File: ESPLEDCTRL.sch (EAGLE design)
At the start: 5 parts, among them J1 22-27-2031-03, X3 ZX62D-B-5PA8

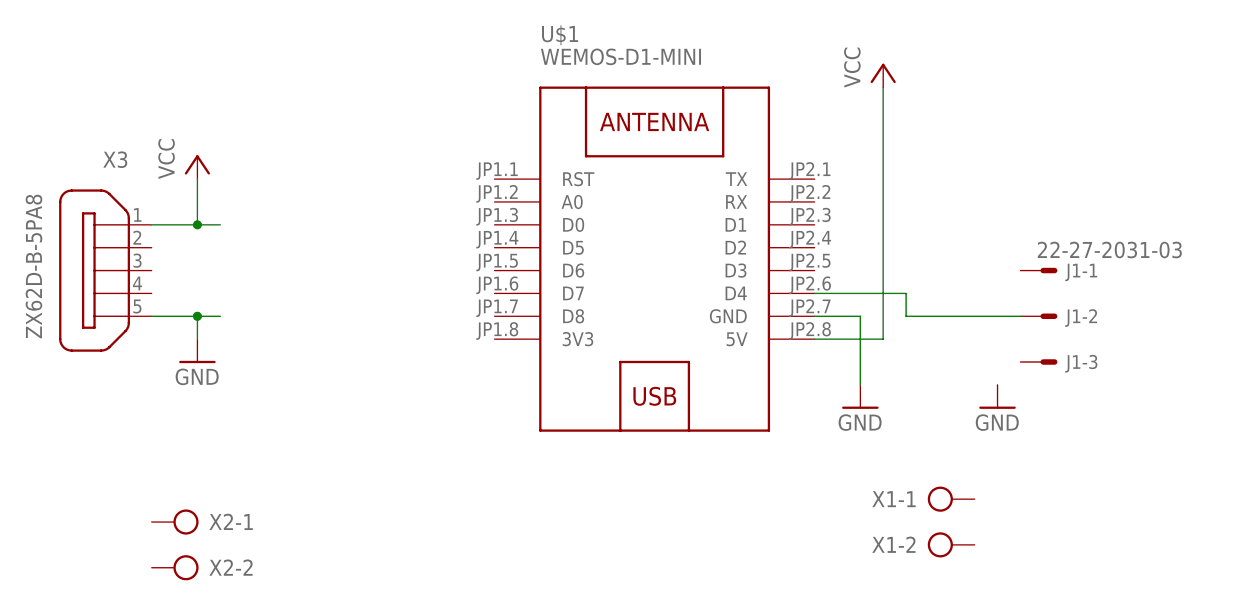
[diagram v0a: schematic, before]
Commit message: bla
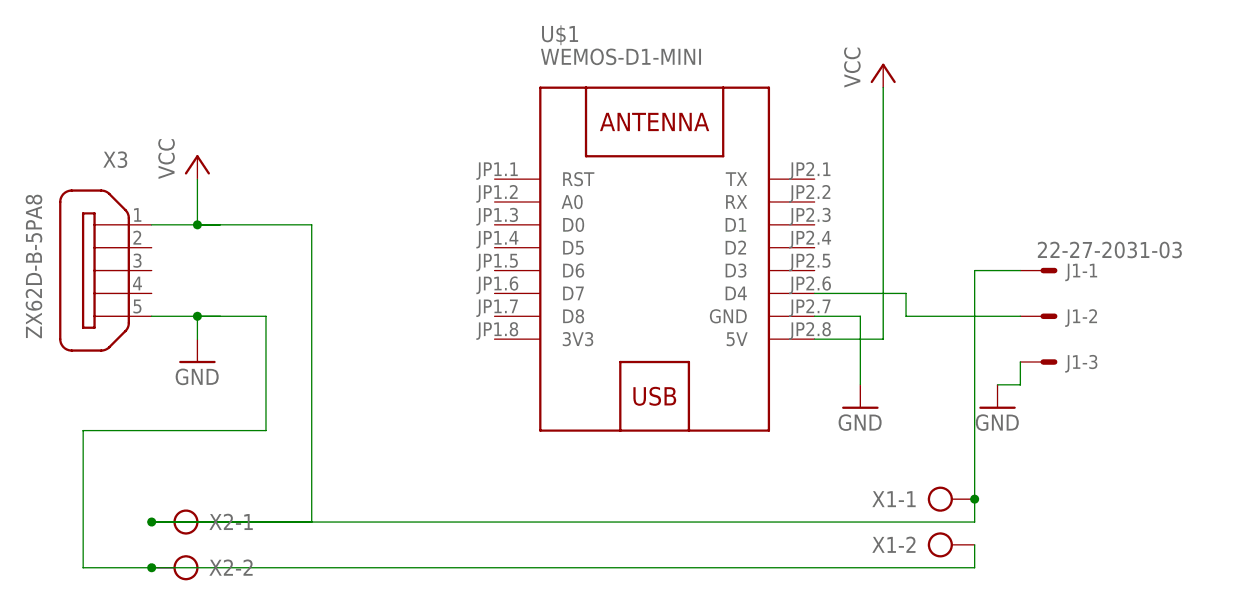
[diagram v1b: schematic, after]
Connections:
- net GND: now also J1-3.S, X1-2.KL, X2-2.KL
- net VCC: now also J1-1.S, X1-1.KL, X2-1.KL
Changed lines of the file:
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@@
 <?xml version="1.0" encoding="utf-8"?>
 <!DOCTYPE eagle SYSTEM "eagle.dtd">
-<eagle version="8.7.1">
+<eagle version="9.5.1">
 <drawing>
 <settings>
@@
 </plain>
 <instances>
-<instance part="X3" gate="G$1" x="27.94" y="58.42" rot="MR0"/>
-<instance part="P+1" gate="VCC" x="38.1" y="71.12"/>
-<instance part="GND1" gate="1" x="38.1" y="48.26"/>
-<instance part="U$1" gate="G$1" x="88.9" y="58.42"/>
-<instance part="X1" gate="-1" x="119.38" y="33.02"/>
-<instance part="X1" gate="-2" x="119.38" y="27.94"/>
-<instance part="X2" gate="-1" x="38.1" y="30.48" rot="MR0"/>
-<instance part="X2" gate="-2" x="38.1" y="25.4" rot="MR0"/>
-<instance part="J1" gate="-1" x="132.08" y="58.42"/>
-<instance part="J1" gate="-2" x="132.08" y="53.34"/>
-<instance part="J1" gate="-3" x="132.08" y="48.26"/>
-<instance part="GND2" gate="1" x="127" y="43.18"/>
-<instance part="P+2" gate="VCC" x="114.3" y="81.28"/>
-<instance part="GND3" gate="1" x="111.76" y="43.18"/>
+<instance part="X3" gate="G$1" x="27.94" y="58.42" smashed="yes" rot="MR0">
+<attribute name="NAME" x="30.48" y="69.85" size="1.778" layer="95" font="vector" rot="MR0"/>
+<attribute name="VALUE" x="19.05" y="50.8" size="1.778" layer="96" font="vector" rot="MR90"/>
+</instance>
+<instance part="P+1" gate="VCC" x="38.1" y="71.12" smashed="yes">
+<attribute name="VALUE" x="35.56" y="68.58" size="1.778" layer="96" rot="R90"/>
+</instance>
+<instance part="GND1" gate="1" x="38.1" y="48.26" smashed="yes">
+<attribute name="VALUE" x="35.56" y="45.72" size="1.778" layer="96"/>
+</instance>
+<instance part="U$1" gate="G$1" x="88.9" y="58.42" smashed="yes">
+<attribute name="NAME" x="76.2" y="83.82" size="1.778" layer="95"/>
+<attribute name="VALUE" x="76.2" y="81.28" size="1.778" layer="96"/>
+</instance>
+<instance part="X1" gate="-1" x="119.38" y="33.02" smashed="yes">
+<attribute name="NAME" x="118.11" y="33.909" size="1.778" layer="95" rot="R180"/>
+</instance>
+<instance part="X1" gate="-2" x="119.38" y="27.94" smashed="yes">
+<attribute name="NAME" x="118.11" y="28.829" size="1.778" layer="95" rot="R180"/>
+<attribute name="VALUE" x="115.57" y="24.257" size="1.778" layer="96"/>
+</instance>
+<instance part="X2" gate="-1" x="38.1" y="30.48" smashed="yes" rot="MR0">
+<attribute name="NAME" x="39.37" y="31.369" size="1.778" layer="95" rot="MR180"/>
+</instance>
+<instance part="X2" gate="-2" x="38.1" y="25.4" smashed="yes" rot="MR0">
+<attribute name="NAME" x="39.37" y="26.289" size="1.778" layer="95" rot="MR180"/>
+<attribute name="VALUE" x="41.91" y="21.717" size="1.778" layer="96" rot="MR0"/>
+</instance>
+<instance part="J1" gate="-1" x="132.08" y="58.42" smashed="yes">
+<attribute name="NAME" x="134.62" y="57.658" size="1.524" layer="95"/>
+<attribute name="VALUE" x="131.318" y="59.817" size="1.778" layer="96"/>
+</instance>
+<instance part="J1" gate="-2" x="132.08" y="53.34" smashed="yes">
+<attribute name="NAME" x="134.62" y="52.578" size="1.524" layer="95"/>
+</instance>
+<instance part="J1" gate="-3" x="132.08" y="48.26" smashed="yes">
+<attribute name="NAME" x="134.62" y="47.498" size="1.524" layer="95"/>
+</instance>
+<instance part="GND2" gate="1" x="127" y="43.18" smashed="yes">
+<attribute name="VALUE" x="124.46" y="40.64" size="1.778" layer="96"/>
+</instance>
+<instance part="P+2" gate="VCC" x="114.3" y="81.28" smashed="yes">
+<attribute name="VALUE" x="111.76" y="78.74" size="1.778" layer="96" rot="R90"/>
+</instance>
+<instance part="GND3" gate="1" x="111.76" y="43.18" smashed="yes">
+<attribute name="VALUE" x="109.22" y="40.64" size="1.778" layer="96"/>
+</instance>
 </instances>
 <busses>
@@
 <net name="GND" class="0">
 <segment>
+<pinref part="GND1" gate="1" pin="GND"/>
 <wire x1="40.64" y1="53.34" x2="38.1" y2="53.34" width="0.1524" layer="91"/>
-<pinref part="GND1" gate="1" pin="GND"/>
 <wire x1="38.1" y1="53.34" x2="38.1" y2="50.8" width="0.1524" layer="91"/>
+<junction x="38.1" y="53.34"/>
 <wire x1="38.1" y1="53.34" x2="33.02" y2="53.34" width="0.1524" layer="91"/>
-<junction x="38.1" y="53.34"/>
 <pinref part="X3" gate="G$1" pin="5"/>
+<pinref part="X1" gate="-2" pin="KL"/>
+<wire x1="33.02" y1="25.4" x2="124.46" y2="25.4" width="0.1524" layer="91"/>
+<wire x1="124.46" y1="25.4" x2="124.46" y2="27.94" width="0.1524" layer="91"/>
+<pinref part="X2" gate="-2" pin="KL"/>
+<wire x1="33.02" y1="25.4" x2="25.4" y2="25.4" width="0.1524" layer="91"/>
+<wire x1="25.4" y1="25.4" x2="25.4" y2="40.64" width="0.1524" layer="91"/>
+<junction x="33.02" y="25.4"/>
+<wire x1="25.4" y1="40.64" x2="45.72" y2="40.64" width="0.1524" layer="91"/>
+<wire x1="45.72" y1="40.64" x2="45.72" y2="53.34" width="0.1524" layer="91"/>
+<wire x1="45.72" y1="53.34" x2="38.1" y2="53.34" width="0.1524" layer="91"/>
 </segment>
 <segment>
@@
 <pinref part="GND3" gate="1" pin="GND"/>
 </segment>
+<segment>
+<pinref part="J1" gate="-3" pin="S"/>
+<pinref part="GND2" gate="1" pin="GND"/>
+<wire x1="129.54" y1="48.26" x2="129.54" y2="45.72" width="0.1524" layer="91"/>
+<wire x1="129.54" y1="45.72" x2="127" y2="45.72" width="0.1524" layer="91"/>
+</segment>
 </net>
 <net name="VCC" class="0">
@@
 <wire x1="40.64" y1="63.5" x2="38.1" y2="63.5" width="0.1524" layer="91"/>
 <wire x1="38.1" y1="63.5" x2="38.1" y2="68.58" width="0.1524" layer="91"/>
+<junction x="38.1" y="63.5"/>
 <wire x1="38.1" y1="63.5" x2="33.02" y2="63.5" width="0.1524" layer="91"/>
-<junction x="38.1" y="63.5"/>
 <pinref part="X3" gate="G$1" pin="1"/>
+<pinref part="X2" gate="-1" pin="KL"/>
+<pinref part="X1" gate="-1" pin="KL"/>
+<wire x1="33.02" y1="30.48" x2="124.46" y2="30.48" width="0.1524" layer="91"/>
+<wire x1="124.46" y1="30.48" x2="124.46" y2="33.02" width="0.1524" layer="91"/>
+<wire x1="38.1" y1="30.48" x2="33.02" y2="30.48" width="0.1524" layer="91"/>
+<junction x="33.02" y="30.48"/>
+<pinref part="J1" gate="-1" pin="S"/>
+<wire x1="129.54" y1="58.42" x2="124.46" y2="58.42" width="0.1524" layer="91"/>
+<wire x1="124.46" y1="58.42" x2="124.46" y2="33.02" width="0.1524" layer="91"/>
+<junction x="124.46" y="33.02"/>
+<wire x1="33.02" y1="30.48" x2="50.8" y2="30.48" width="0.1524" layer="91"/>
+<wire x1="50.8" y1="30.48" x2="50.8" y2="63.5" width="0.1524" layer="91"/>
+<wire x1="50.8" y1="63.5" x2="38.1" y2="63.5" width="0.1524" layer="91"/>
 </segment>
 <segment>

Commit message: Eine Diode
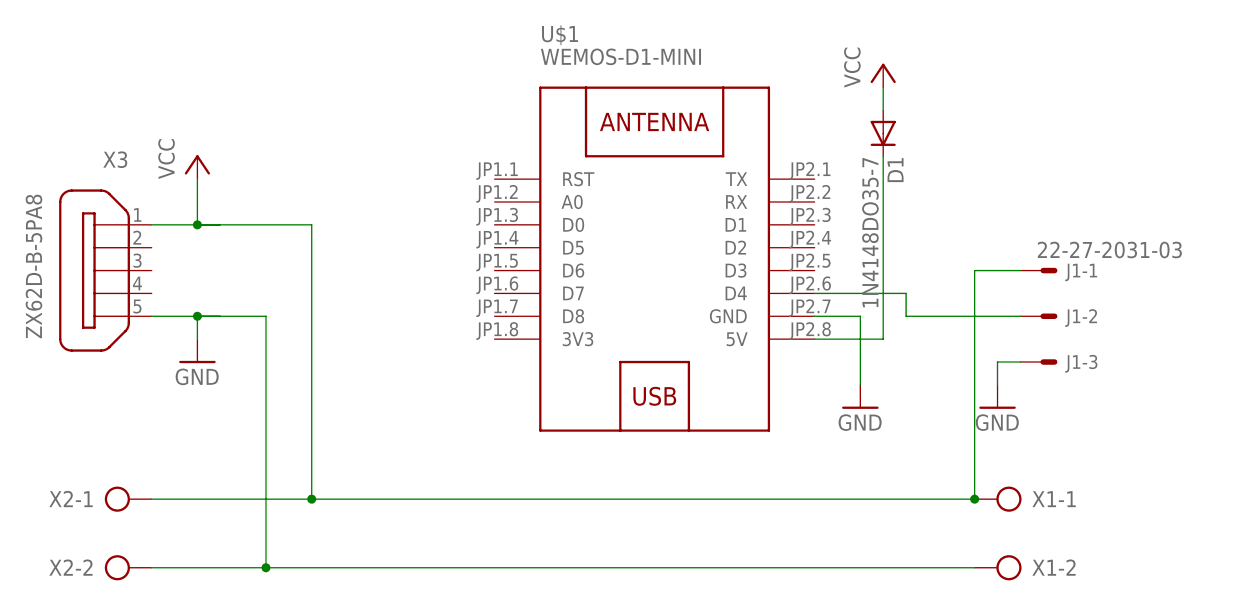
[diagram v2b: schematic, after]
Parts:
- added D1: 1N4148DO35-7, diode:1N4148DO35-7
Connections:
- new net N$2: D1.C, U$1.5V
- net VCC: now also D1.A; no longer U$1.5V
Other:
- moved on the sheet: X1-1, X1-2, X2-1, X2-2
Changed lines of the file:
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@@
 <?xml version="1.0" encoding="utf-8"?>
 <!DOCTYPE eagle SYSTEM "eagle.dtd">
-<eagle version="9.5.1">
+<eagle version="8.7.1">
 <drawing>
 <settings>
@@
 <part name="P+2" library="supply1" library_urn="urn:adsk.eagle:library:371" deviceset="VCC" device=""/>
 <part name="GND3" library="supply1" library_urn="urn:adsk.eagle:library:371" deviceset="GND" device=""/>
+<part name="D1" library="diode" library_urn="urn:adsk.eagle:library:210" deviceset="1N4148" device="DO35-7" package3d_urn="urn:adsk.eagle:package:43339/1"/>
 </parts>
 <sheets>
@@
 <attribute name="VALUE" x="76.2" y="81.28" size="1.778" layer="96"/>
 </instance>
-<instance part="X1" gate="-1" x="119.38" y="33.02" smashed="yes">
-<attribute name="NAME" x="118.11" y="33.909" size="1.778" layer="95" rot="R180"/>
-</instance>
-<instance part="X1" gate="-2" x="119.38" y="27.94" smashed="yes">
-<attribute name="NAME" x="118.11" y="28.829" size="1.778" layer="95" rot="R180"/>
-<attribute name="VALUE" x="115.57" y="24.257" size="1.778" layer="96"/>
-</instance>
-<instance part="X2" gate="-1" x="38.1" y="30.48" smashed="yes" rot="MR0">
-<attribute name="NAME" x="39.37" y="31.369" size="1.778" layer="95" rot="MR180"/>
-</instance>
-<instance part="X2" gate="-2" x="38.1" y="25.4" smashed="yes" rot="MR0">
-<attribute name="NAME" x="39.37" y="26.289" size="1.778" layer="95" rot="MR180"/>
-<attribute name="VALUE" x="41.91" y="21.717" size="1.778" layer="96" rot="MR0"/>
+<instance part="X1" gate="-1" x="129.54" y="33.02" smashed="yes" rot="R180">
+<attribute name="NAME" x="130.81" y="32.131" size="1.778" layer="95"/>
+</instance>
+<instance part="X1" gate="-2" x="129.54" y="25.4" smashed="yes" rot="R180">
+<attribute name="NAME" x="130.81" y="24.511" size="1.778" layer="95"/>
+<attribute name="VALUE" x="133.35" y="29.083" size="1.778" layer="96" rot="R180"/>
+</instance>
+<instance part="X2" gate="-1" x="27.94" y="33.02" smashed="yes" rot="MR180">
+<attribute name="NAME" x="26.67" y="32.131" size="1.778" layer="95" rot="MR0"/>
+</instance>
+<instance part="X2" gate="-2" x="27.94" y="25.4" smashed="yes" rot="MR180">
+<attribute name="NAME" x="26.67" y="24.511" size="1.778" layer="95" rot="MR0"/>
+<attribute name="VALUE" x="24.13" y="29.083" size="1.778" layer="96" rot="MR180"/>
 </instance>
 <instance part="J1" gate="-1" x="132.08" y="58.42" smashed="yes">
@@
 <attribute name="VALUE" x="109.22" y="40.64" size="1.778" layer="96"/>
 </instance>
+<instance part="D1" gate="G$1" x="114.3" y="73.66" rot="R270"/>
 </instances>
 <busses>
@@
 <pinref part="X3" gate="G$1" pin="5"/>
 <pinref part="X1" gate="-2" pin="KL"/>
-<wire x1="33.02" y1="25.4" x2="124.46" y2="25.4" width="0.1524" layer="91"/>
-<wire x1="124.46" y1="25.4" x2="124.46" y2="27.94" width="0.1524" layer="91"/>
+<wire x1="33.02" y1="25.4" x2="45.72" y2="25.4" width="0.1524" layer="91"/>
 <pinref part="X2" gate="-2" pin="KL"/>
-<wire x1="33.02" y1="25.4" x2="25.4" y2="25.4" width="0.1524" layer="91"/>
-<wire x1="25.4" y1="25.4" x2="25.4" y2="40.64" width="0.1524" layer="91"/>
-<junction x="33.02" y="25.4"/>
-<wire x1="25.4" y1="40.64" x2="45.72" y2="40.64" width="0.1524" layer="91"/>
-<wire x1="45.72" y1="40.64" x2="45.72" y2="53.34" width="0.1524" layer="91"/>
+<wire x1="45.72" y1="25.4" x2="124.46" y2="25.4" width="0.1524" layer="91"/>
+<wire x1="45.72" y1="25.4" x2="45.72" y2="53.34" width="0.1524" layer="91"/>
 <wire x1="45.72" y1="53.34" x2="38.1" y2="53.34" width="0.1524" layer="91"/>
+<junction x="45.72" y="25.4"/>
 </segment>
 <segment>
@@
 <pinref part="J1" gate="-3" pin="S"/>
 <pinref part="GND2" gate="1" pin="GND"/>
-<wire x1="129.54" y1="48.26" x2="129.54" y2="45.72" width="0.1524" layer="91"/>
-<wire x1="129.54" y1="45.72" x2="127" y2="45.72" width="0.1524" layer="91"/>
+<wire x1="129.54" y1="48.26" x2="127" y2="48.26" width="0.1524" layer="91"/>
+<wire x1="127" y1="48.26" x2="127" y2="45.72" width="0.1524" layer="91"/>
 </segment>
 </net>
@@
 <wire x1="38.1" y1="63.5" x2="33.02" y2="63.5" width="0.1524" layer="91"/>
 <pinref part="X3" gate="G$1" pin="1"/>
-<pinref part="X2" gate="-1" pin="KL"/>
 <pinref part="X1" gate="-1" pin="KL"/>
-<wire x1="33.02" y1="30.48" x2="124.46" y2="30.48" width="0.1524" layer="91"/>
-<wire x1="124.46" y1="30.48" x2="124.46" y2="33.02" width="0.1524" layer="91"/>
-<wire x1="38.1" y1="30.48" x2="33.02" y2="30.48" width="0.1524" layer="91"/>
-<junction x="33.02" y="30.48"/>
 <pinref part="J1" gate="-1" pin="S"/>
+<wire x1="50.8" y1="33.02" x2="124.46" y2="33.02" width="0.1524" layer="91"/>
 <wire x1="129.54" y1="58.42" x2="124.46" y2="58.42" width="0.1524" layer="91"/>
 <wire x1="124.46" y1="58.42" x2="124.46" y2="33.02" width="0.1524" layer="91"/>
 <junction x="124.46" y="33.02"/>
-<wire x1="33.02" y1="30.48" x2="50.8" y2="30.48" width="0.1524" layer="91"/>
-<wire x1="50.8" y1="30.48" x2="50.8" y2="63.5" width="0.1524" layer="91"/>
+<wire x1="50.8" y1="33.02" x2="50.8" y2="63.5" width="0.1524" layer="91"/>
 <wire x1="50.8" y1="63.5" x2="38.1" y2="63.5" width="0.1524" layer="91"/>
-</segment>
-<segment>
-<pinref part="U$1" gate="G$1" pin="5V"/>
-<wire x1="106.68" y1="50.8" x2="114.3" y2="50.8" width="0.1524" layer="91"/>
+<pinref part="X2" gate="-1" pin="KL"/>
+<wire x1="50.8" y1="33.02" x2="33.02" y2="33.02" width="0.1524" layer="91"/>
+<junction x="50.8" y="33.02"/>
+</segment>
+<segment>
 <pinref part="P+2" gate="VCC" pin="VCC"/>
-<wire x1="114.3" y1="50.8" x2="114.3" y2="78.74" width="0.1524" layer="91"/>
+<pinref part="D1" gate="G$1" pin="A"/>
+<wire x1="114.3" y1="76.2" x2="114.3" y2="78.74" width="0.1524" layer="91"/>
 </segment>
 </net>
@@
 </segment>
 </net>
+<net name="N$2" class="0">
+<segment>
+<pinref part="U$1" gate="G$1" pin="5V"/>
+<wire x1="106.68" y1="50.8" x2="114.3" y2="50.8" width="0.1524" layer="91"/>
+<wire x1="114.3" y1="50.8" x2="114.3" y2="71.12" width="0.1524" layer="91"/>
+<pinref part="D1" gate="G$1" pin="C"/>
+</segment>
+</net>
